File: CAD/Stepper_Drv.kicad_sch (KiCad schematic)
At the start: 28 parts, among them U1 SN74F125DR, U14 SN74LVC4245APW, U2 SN74F125DR, U21 SN74F125DR, U22 SN74F125DR, U25 SN74LVC4245APW, U26 SN74LVC4245APW, U6 SN74F125DR

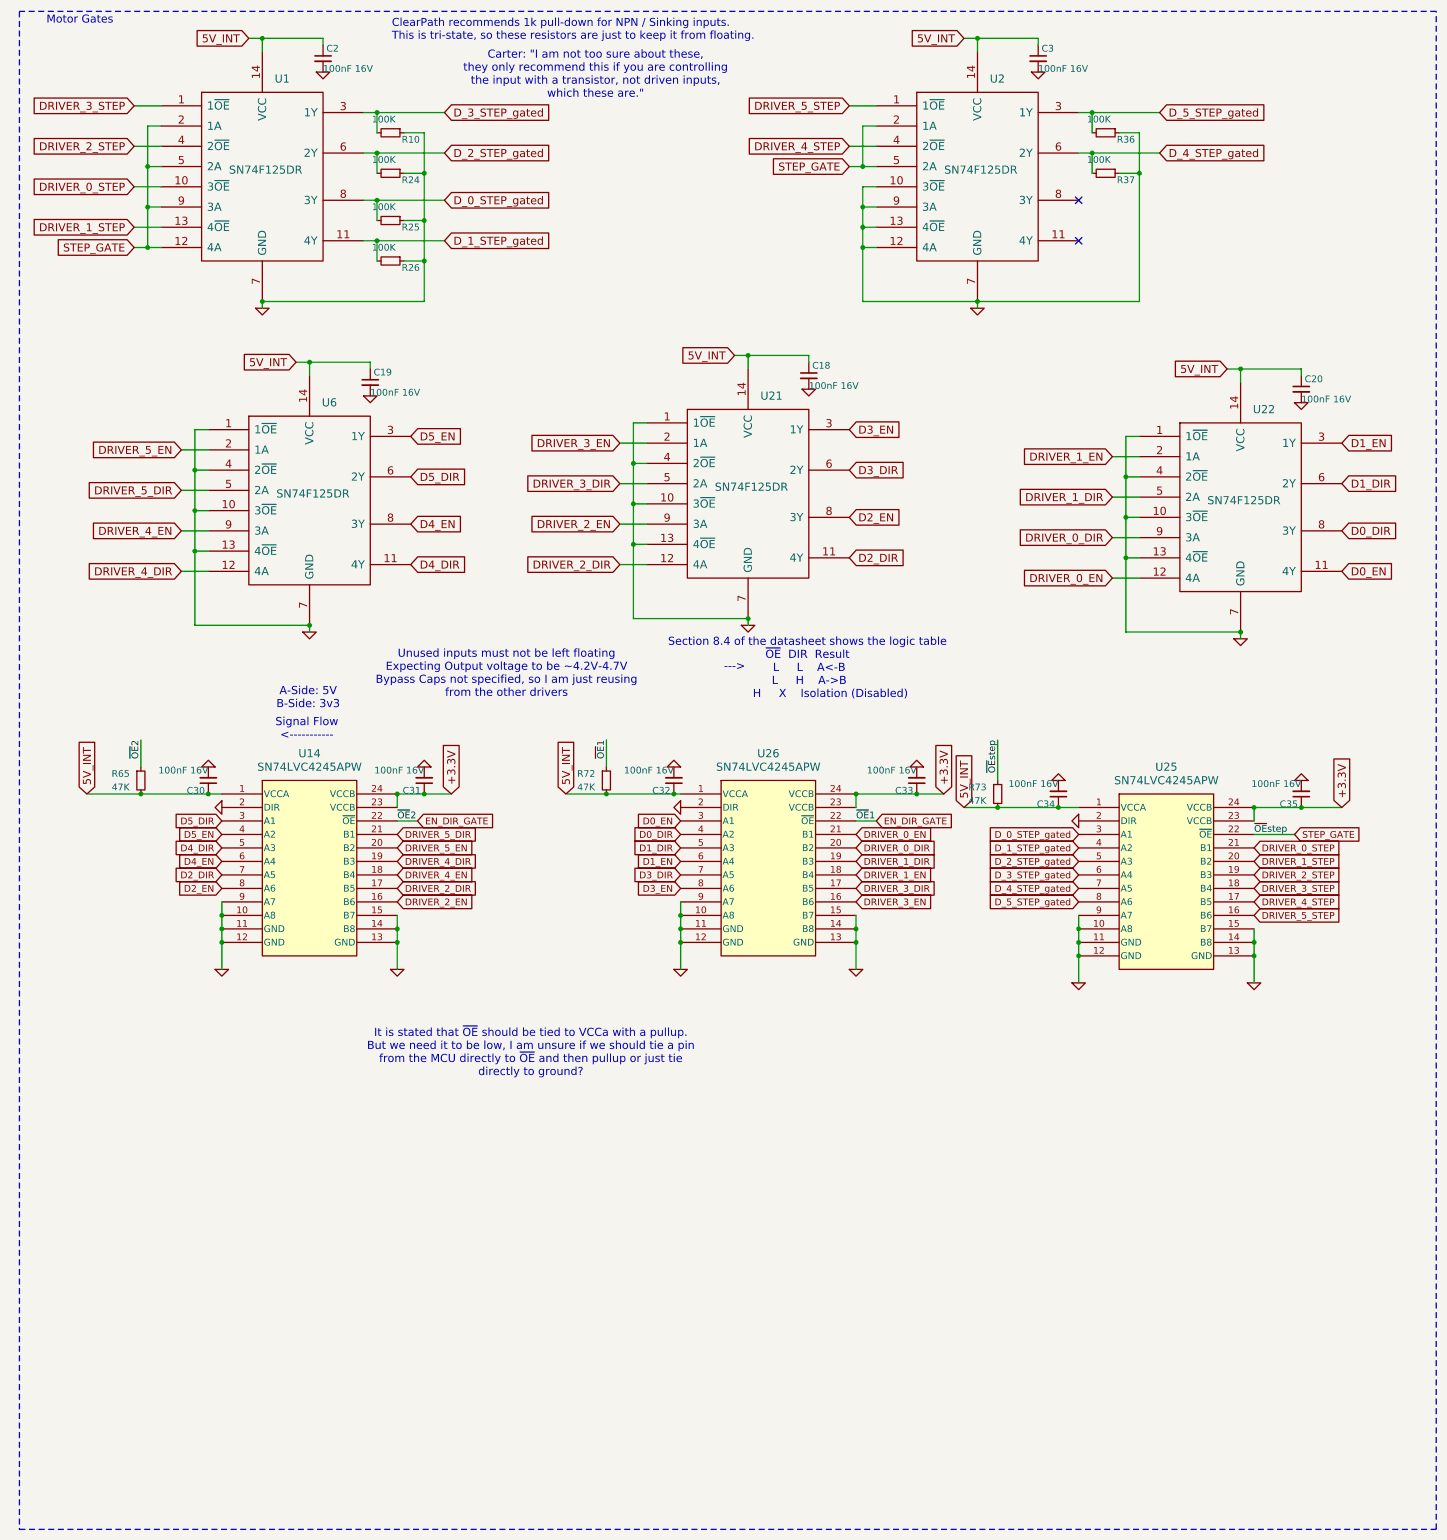
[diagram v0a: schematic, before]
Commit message: 12 Unconnected left
Almost done :) Brian fried
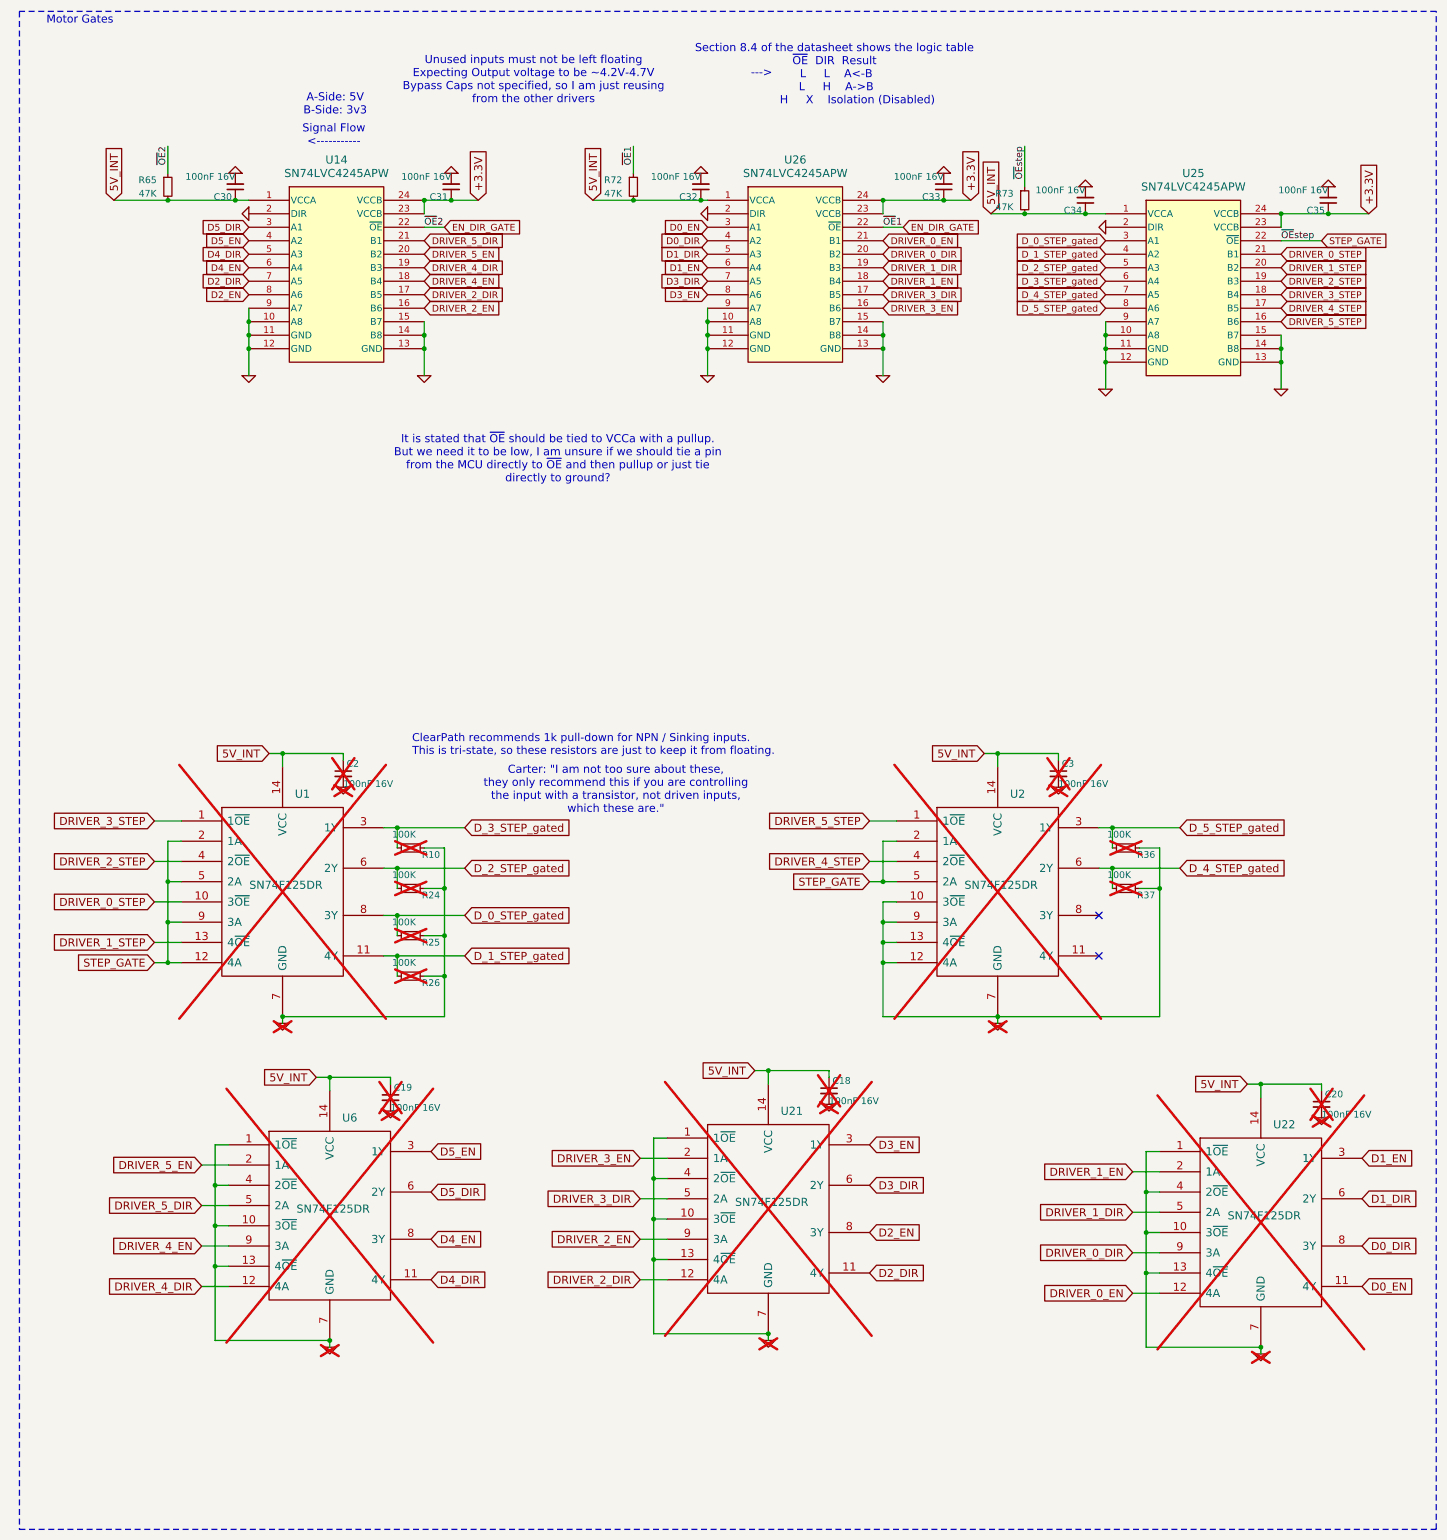
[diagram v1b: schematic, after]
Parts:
- C18, C19, C2, C20, C3, R10, R24, R25, R26, R36, R37, U1, U2, U21, U22, U6: now not fitted; now left out of the parts list
- R65, R72, R73: footprint Resistor_SMD:R_0402_1005Metric_Wbry -> Resistor_SMD:R_0402_1005Metric
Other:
- moved on the sheet: C30, C31, C32, C33, C34, C35, R65, R72, R73, U14, U25, U26
